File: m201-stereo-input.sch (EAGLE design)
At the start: 83 parts, among them U1 FX2-20P-1.27DS, U2 FX2-20S-1.27DS, U3 ERM1-5MM

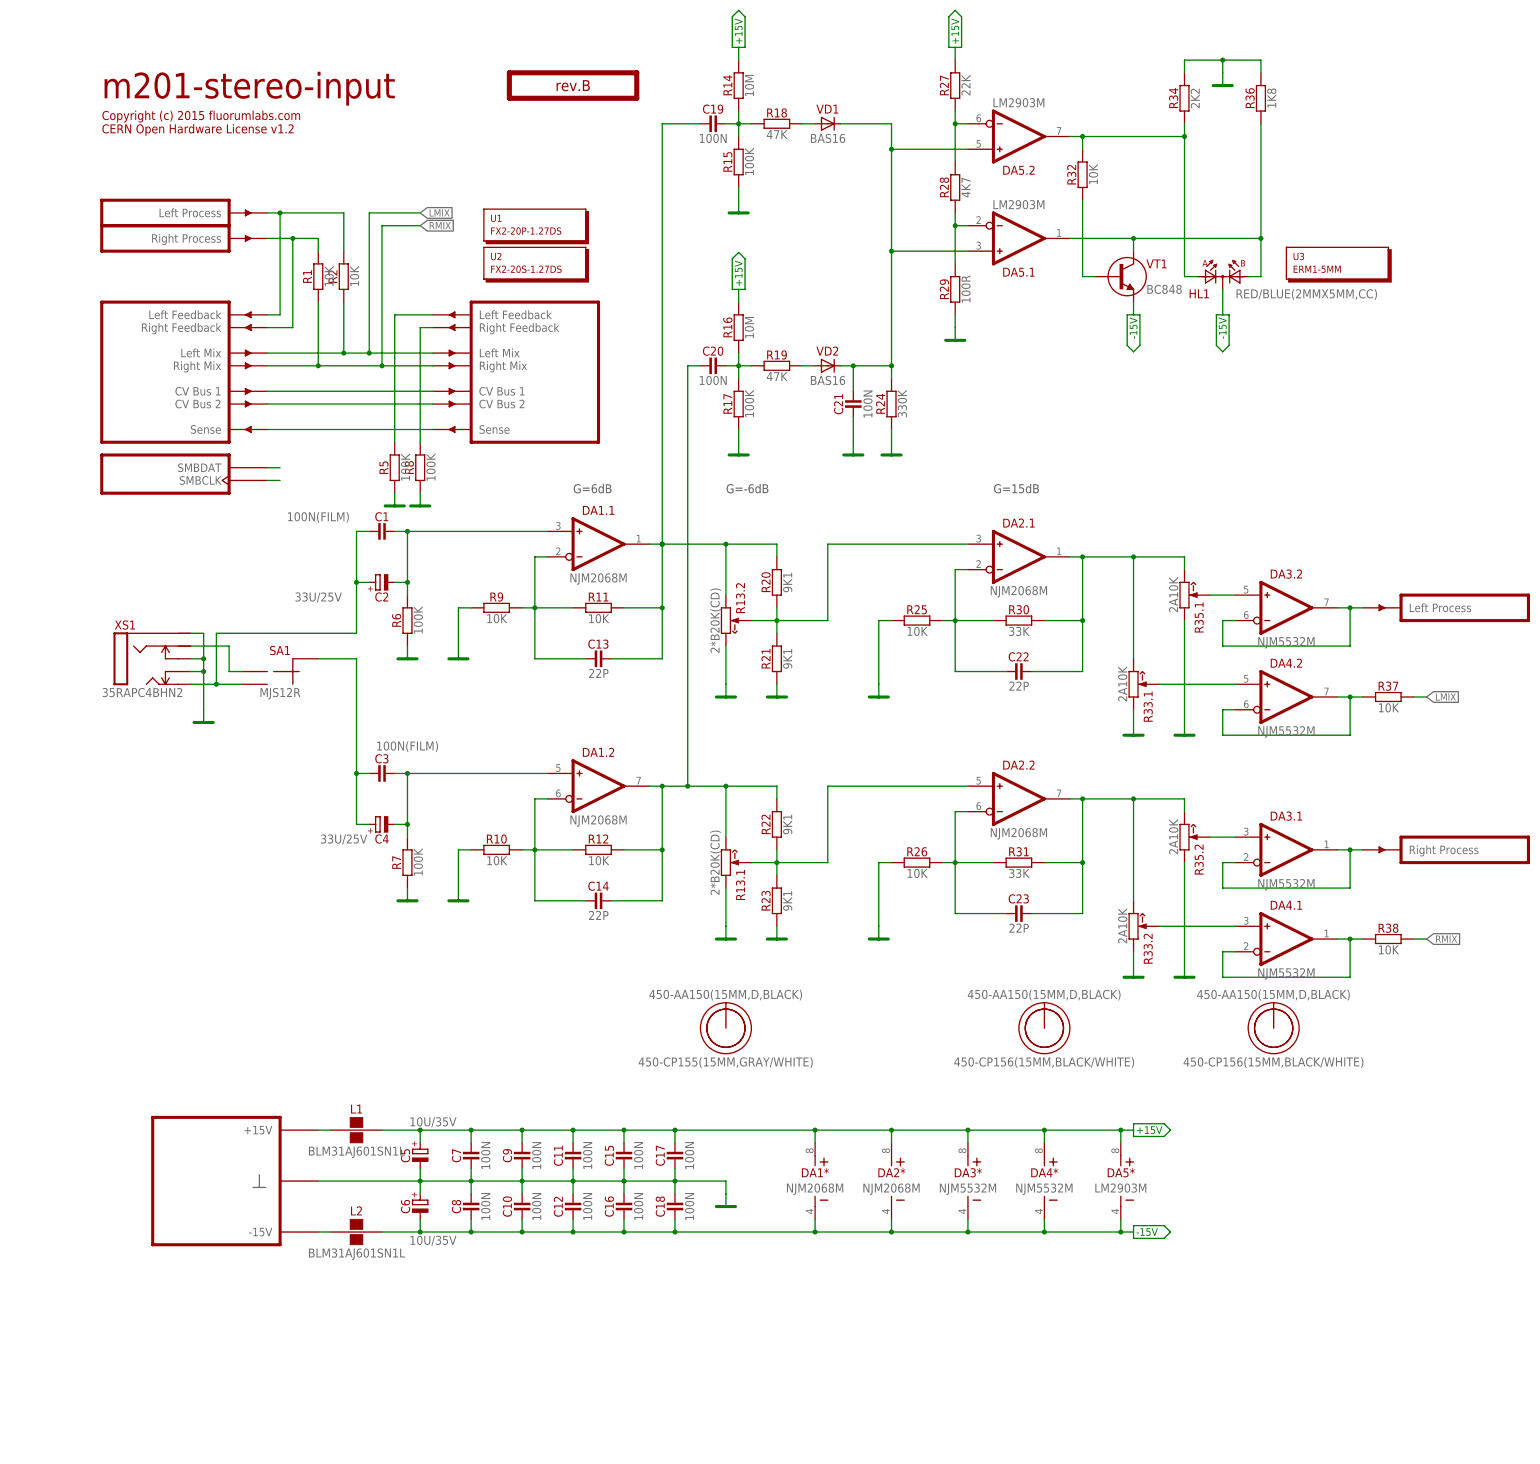
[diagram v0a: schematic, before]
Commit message: M201 In T/H
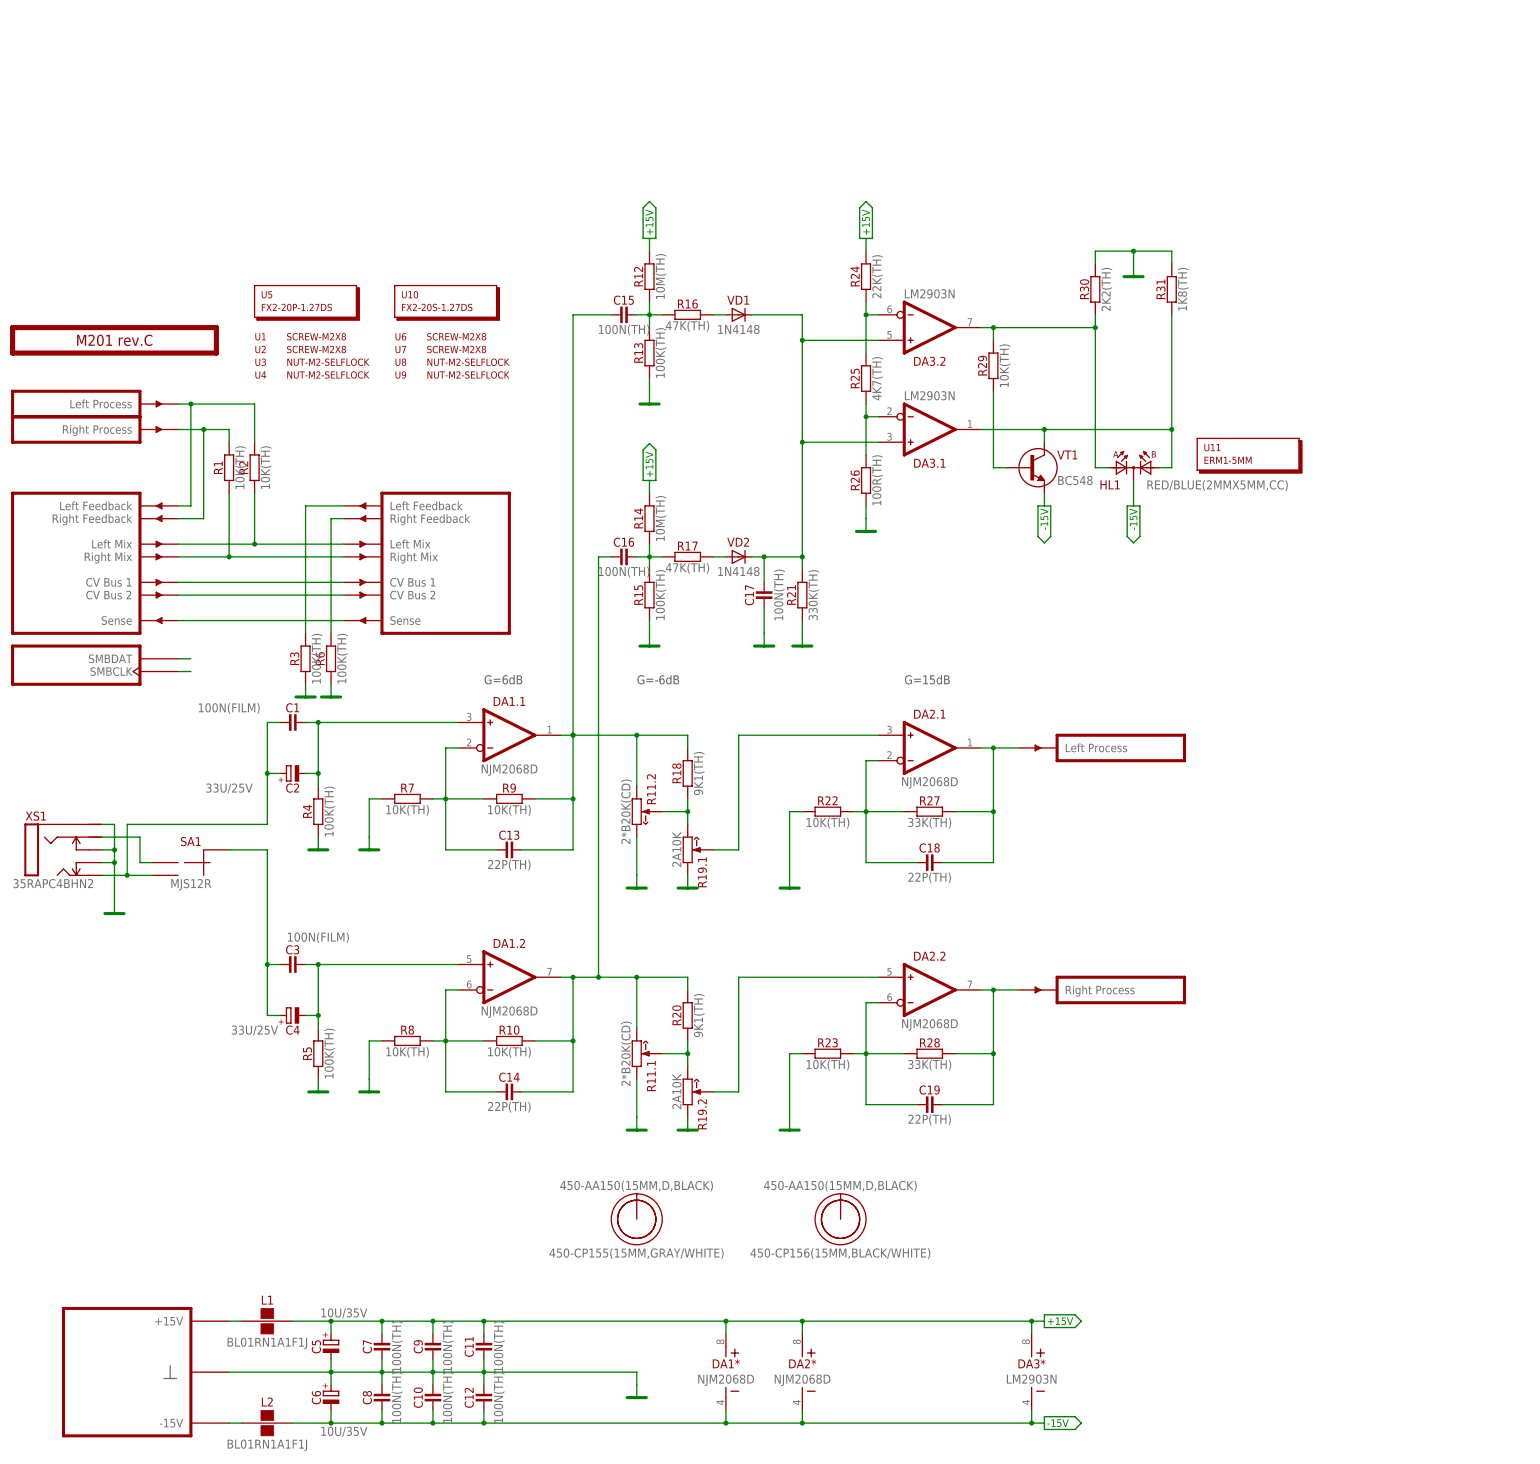
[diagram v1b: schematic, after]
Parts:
- removed C20, C21: 100N, capacitors:100N
- removed C22, C23: 22P, capacitors:22P
- removed DA4: NJM5532M, ic-jrc:NJM5532M
- removed DA5: LM2903M, ic-fairchild:LM2903M
- removed O5, O7: 450-CP156(15MM,BLACK/WHITE), hardware:450-CP156(15MM,BLACK/WHITE)
- removed O6: 450-AA150(15MM,D,BLACK), hardware:450-AA150(15MM,D,BLACK)
- removed R32, R37, R38: 10K, resistors:10K
- removed R33, R35: 2A10K, potentiometers:2A10K
- removed R34: 2K2, resistors:2K2
- removed R36: 1K8, resistors:1K8
- added R3, R4: 100K(TH), resistors:100K(TH)
- added U10: FX2-20S-1.27DS, hardware:FX2-20S-1.27DS
- added U11: ERM1-5MM, hardware:ERM1-5MM
- added U4, U8, U9: NUT-M2-SELFLOCK, hardware:NUT-M2-SELFLOCK
- added U5: FX2-20P-1.27DS, hardware:FX2-20P-1.27DS
- added U6, U7: SCREW-M2X8, hardware:SCREW-M2X8
- C10, C11, C12, C15, C16, C17, C7, C8, C9: value 100N -> 100N(TH); device capacitors:100N -> capacitors:100N(TH)
- C13, C14: value 22P -> 22P(TH); device capacitors:22P -> capacitors:22P(TH)
- C18, C19: value 100N -> 22P(TH); device capacitors:100N -> capacitors:22P(TH)
- DA1, DA2: value NJM2068M -> NJM2068D; device ic-jrc:NJM2068M -> ic-jrc:NJM2068D
- DA3: value NJM5532M -> LM2903N; device ic-jrc:NJM5532M -> ic-fairchild:LM2903N
- L1, L2: value BLM31AJ601SN1L -> BL01RN1A1F1J; device inductors:BLM31AJ601SN1L -> inductors:BL01RN1A1F1J
- O1: value (none) -> 450-AA150(15MM,D,BLACK); device text:TITLE -> hardware:450-AA150(15MM,D,BLACK)
- O2: value 450-AA150(15MM,D,BLACK) -> 450-CP155(15MM,GRAY/WHITE); device hardware:450-AA150(15MM,D,BLACK) -> hardware:450-CP155(15MM,GRAY/WHITE)
- O3: value 450-CP155(15MM,GRAY/WHITE) -> 450-AA150(15MM,D,BLACK); device hardware:450-CP155(15MM,GRAY/WHITE) -> hardware:450-AA150(15MM,D,BLACK)
- O4: value 450-AA150(15MM,D,BLACK) -> 450-CP156(15MM,BLACK/WHITE); device hardware:450-AA150(15MM,D,BLACK) -> hardware:450-CP156(15MM,BLACK/WHITE)
- PCB1: value rev.B -> M201 rev.C
- R1, R10, R2, R9: value 10K -> 10K(TH); device resistors:10K -> resistors:10K(TH)
- R11: value 10K -> 2*B20K(CD); device resistors:10K -> potentiometers:2B20K(CD)
- R12: value 10K -> 10M(TH); device resistors:10K -> resistors:10M(TH)
- R13: value 2*B20K(CD) -> 100K(TH); device potentiometers:2B20K(CD) -> resistors:100K(TH)
- R14: value 10M -> 10M(TH); device resistors:10M -> resistors:10M(TH)
- R15, R5, R6: value 100K -> 100K(TH); device resistors:100K -> resistors:100K(TH)
- R16: value 10M -> 47K(TH); device resistors:10M -> resistors:47K(TH)
- R17: value 100K -> 47K(TH); device resistors:100K -> resistors:47K(TH)
- R18: value 47K -> 9K1(TH); device resistors:47K -> resistors:9K1(TH)
- R19: value 47K -> 2A10K; device resistors:47K -> potentiometers:2A10K
- R20: value 9K1 -> 9K1(TH); device resistors:9K1 -> resistors:9K1(TH)
- R21: value 9K1 -> 330K(TH); device resistors:9K1 -> resistors:330K(TH)
- R22, R23: value 9K1 -> 10K(TH); device resistors:9K1 -> resistors:10K(TH)
- R24: value 330K -> 22K(TH); device resistors:330K -> resistors:22K(TH)
- R25: value 10K -> 4K7(TH); device resistors:10K -> resistors:4K7(TH)
- R26: value 10K -> 100R(TH); device resistors:10K -> resistors:100R(TH)
- R27: value 22K -> 33K(TH); device resistors:22K -> resistors:33K(TH)
- R28: value 4K7 -> 33K(TH); device resistors:4K7 -> resistors:33K(TH)
- R29: value 100R -> 10K(TH); device resistors:100R -> resistors:10K(TH)
- R30: value 33K -> 2K2(TH); device resistors:33K -> resistors:2K2(TH)
- R31: value 33K -> 1K8(TH); device resistors:33K -> resistors:1K8(TH)
- R7, R8: value 100K -> 10K(TH); device resistors:100K -> resistors:10K(TH)
- U1: value FX2-20P-1.27DS -> SCREW-M2X8; device hardware:FX2-20P-1.27DS -> hardware:SCREW-M2X8
- U2: value FX2-20S-1.27DS -> SCREW-M2X8; device hardware:FX2-20S-1.27DS -> hardware:SCREW-M2X8
- U3: value ERM1-5MM -> NUT-M2-SELFLOCK; device hardware:ERM1-5MM -> hardware:NUT-M2-SELFLOCK
- VD1, VD2: value BAS16 -> 1N4148; device diodes:BAS16 -> diodes:1N4148
- VT1: value BC848 -> BC548; device transistors-npn:BC848 -> transistors-npn:BC548
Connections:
- removed net N$18: DA3.2.IN-, DA3.2.OUT, PCB1G$4.OUTL
- removed net N$20: DA4.2.IN-, DA4.2.OUT, R37.1
- removed net N$21: DA3.1.IN-, DA3.1.OUT, PCB1G$5.OUTR
- removed net N$22: DA4.1.IN-, DA4.1.OUT, R38.1
- removed net N$23: DA3.2.IN+, R35.1.W
- removed net N$24: DA4.2.IN+, R33.1.W
- removed net N$25: DA3.1.IN+, R35.2.W
- removed net N$28: DA4.1.IN+, R33.2.W
- new net N$30: R11.2.W, R18.1, R19.1.CW
- new net N$32: R11.1.W, R19.2.CW, R20.1
- net +15V: now also R12.2, R24.2; no longer C15.2, C17.2, DA4*.V+, DA5*.V+, R16.2, R27.2
- net -15V: no longer C16.1, C18.1, DA4*.V-, DA5*.V-
- net GND: now also R11.1.CCW, R11.2.CW, R13.1, R19.1.CCW, R19.2.CCW, R22.1, R3.1, R30.2, R31.2, R4.1; no longer C15.1, C16.2, C18.2, C21.1, R10.1, R13.1.CCW, R13.2.CW, R17.1, R24.1, R25.1, R29.1, R33.1.CCW, R33.2.CCW, R34.2, R35.1.CCW, R35.2.CCW, R36.2, R9.1
- net LMIX: no longer R37.2
- net N$10: now also R4.2; no longer R6.2
- net N$11: now also C19.2, PCB1G$5.OUTR, R28.2; no longer C23.2, R31.2, R33.2.CW, R35.2.CW
- net N$12: now also C18.2, PCB1G$4.OUTL, R27.2; no longer C22.2, R30.2, R33.1.CW, R35.1.CW
- net N$13: now also C18.1, R22.2, R27.1; no longer C22.1, R25.2, R30.1
- net N$14: now also C19.1, R23.2, R28.1; no longer C23.1, R26.2, R31.1
- net N$15: now also C16.1, R10.2, R11.1.CW, R20.2; no longer C20.1, R12.2, R13.1.CW, R22.2
- net N$17: now also C15.2, R12.1, R13.2, R16.1; no longer C19.2, R14.1, R15.2, R18.1
- net N$19: now also C15.1, R11.2.CCW, R18.2, R9.2; no longer C19.1, R11.2, R13.2.CCW, R20.2
- net N$2: now also R6.2; no longer R8.2
- net N$26: now also R7.2, R9.1; no longer R11.1, R9.2
- net N$27: now also R10.1, R8.2; no longer R10.2, R12.1
- net N$29: now also R16.2; no longer R18.2
- net N$3: now also R19.1.W; no longer R13.2.W, R20.1, R21.2
- net N$31: now also C16.2, R14.1, R15.2, R17.1; no longer C20.2, R16.1, R17.2, R19.1
- net N$4: now also R3.2; no longer R5.2
- net N$44: now also R17.2; no longer R19.2
- net N$45: now also C17.2, DA3.1.IN+, DA3.2.IN+, R21.2; no longer C21.2, DA5.1.IN+, DA5.2.IN+, R24.2
- net N$46: now also DA3.1.IN-, R25.1, R26.2; no longer DA5.1.IN-, R28.1, R29.2
- net N$47: now also DA3.2.IN-, R24.1, R25.2; no longer DA5.2.IN-, R27.1, R28.2
- net N$48: now also DA3.2.OUT, R29.2, R30.1; no longer DA5.2.OUT, R32.2, R34.1
- net N$49: now also R29.1; no longer R32.1
- net N$51: now also DA3.1.OUT, R31.1; no longer DA5.1.OUT, R36.1
- net N$8: now also R19.2.W; no longer R13.1.W, R22.1, R23.2
- net N$9: now also R5.2; no longer R7.2
- net RMIX: no longer R38.2
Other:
- moved on the sheet: C1, C10, C11, C12, C13, C14, C15, C16, C17, C18, C19, C2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
